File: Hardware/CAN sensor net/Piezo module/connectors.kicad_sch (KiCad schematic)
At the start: 7 parts, among them J1 532610671, J2 532610671, J3 USB_B_Micro, U4 USBLC6-2SC6

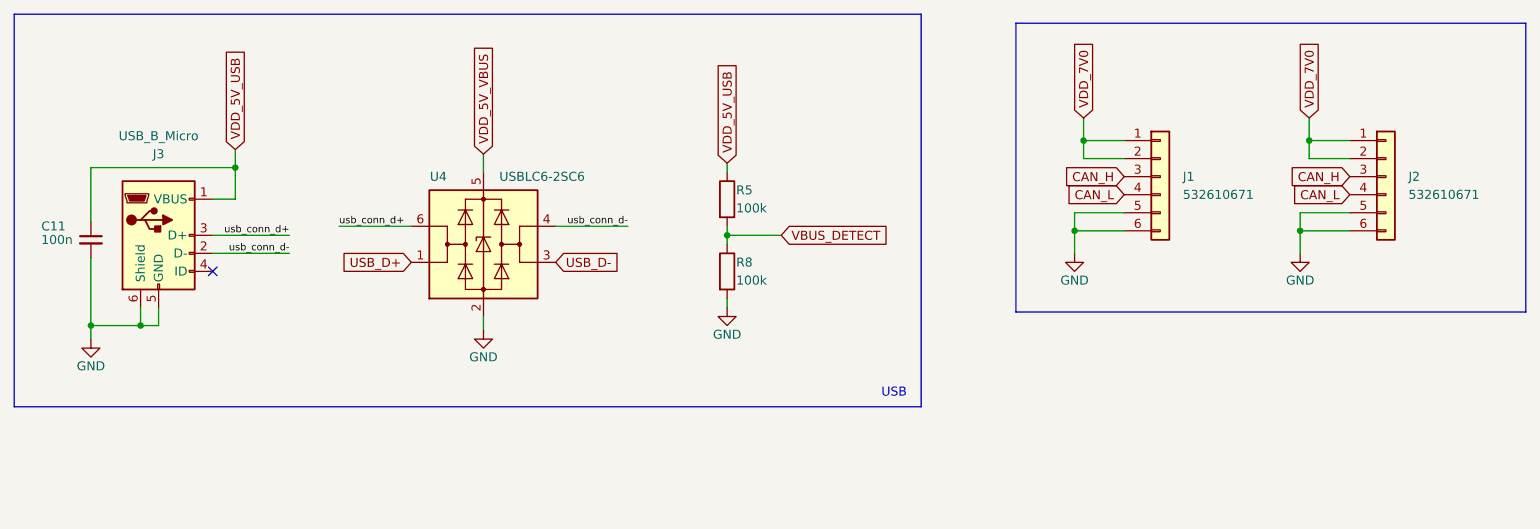
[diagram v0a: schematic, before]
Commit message: Bugfix
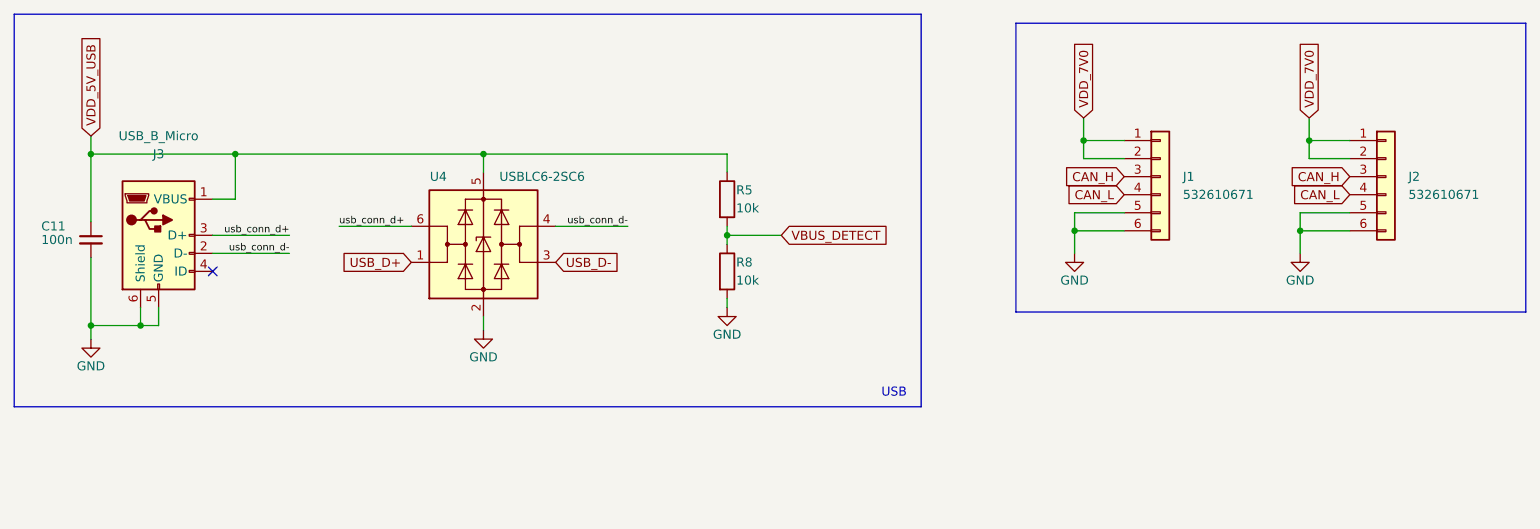
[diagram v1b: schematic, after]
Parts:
- R5, R8: value 100k -> 10k
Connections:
- net VDD_5V_VBUS is gone; now on net VDD_5V_USB: U4.5 (VBUS)
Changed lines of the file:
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@@
 	(paper "A4")
 	(junction
-		(at 52.705 43.815)
+		(at 52.705 41.91)
+		(diameter 0)
+		(color 0 0 0 0)
+	)
+	(junction
+		(at 32.385 41.91)
+		(diameter 0)
+		(color 0 0 0 0)
+	)
+	(junction
+		(at 87.63 41.91)
 		(diameter 0)
 		(color 0 0 0 0)
@@
 	(wire
 		(pts
-			(xy 121.92 43.18) (xy 121.92 44.45)
+			(xy 121.92 41.91) (xy 121.92 44.45)
 		)
 		(stroke
@@
 		)
 	)
+	(wire
+		(pts
+			(xy 52.705 41.91) (xy 87.63 41.91)
+		)
+		(stroke
+			(width 0)
+			(type default)
+		)
+	)
 	(polyline
 		(pts
@@
 	(wire
 		(pts
-			(xy 52.705 48.26) (xy 52.705 43.815)
+			(xy 52.705 41.91) (xy 52.705 48.26)
 		)
 		(stroke
@@
 	(wire
 		(pts
+			(xy 121.92 41.91) (xy 87.63 41.91)
+		)
+		(stroke
+			(width 0)
+			(type default)
+		)
+	)
+	(wire
+		(pts
 			(xy 87.63 64.77) (xy 87.63 66.675)
 		)
@@
 	(wire
 		(pts
-			(xy 52.705 41.275) (xy 52.705 43.815)
+			(xy 32.385 39.37) (xy 32.385 41.91)
 		)
 		(stroke
@@
 	(wire
 		(pts
-			(xy 52.705 43.815) (xy 32.385 43.815)
+			(xy 52.705 41.91) (xy 32.385 41.91)
 		)
 		(stroke
@@
 	(wire
 		(pts
-			(xy 32.385 43.815) (xy 32.385 51.435)
+			(xy 32.385 41.91) (xy 32.385 51.435)
 		)
 		(stroke
@@
 	(global_label "VDD_5V_USB"
 		(shape input)
-		(at 121.92 43.18 90)
+		(at 32.385 39.37 90)
 		(fields_autoplaced yes)
 		(effects
@@
 		)
 		(property "Intersheetrefs" "${INTERSHEET_REFS}"
-			(at 121.92 28.5229 90)
-			(effects
-				(font
-					(size 1.27 1.27)
-				)
-				(justify left)
-				(hide yes)
-			)
-		)
-	)
-	(global_label "VDD_5V_USB"
-		(shape input)
-		(at 52.705 41.275 90)
-		(fields_autoplaced yes)
-		(effects
-			(font
-				(size 1.27 1.27)
-			)
-			(justify left)
-		)
-		(property "Intersheetrefs" "${INTERSHEET_REFS}"
-			(at 52.705 26.6179 90)
-			(effects
-				(font
-					(size 1.27 1.27)
-				)
-				(justify left)
-				(hide yes)
-			)
-		)
-	)
-	(global_label "VDD_5V_VBUS"
-		(shape input)
-		(at 87.63 41.91 90)
-		(fields_autoplaced yes)
-		(effects
-			(font
-				(size 1.27 1.27)
-			)
-			(justify left)
-		)
-		(property "Intersheetrefs" "${INTERSHEET_REFS}"
-			(at 87.7094 26.7364 90)
+			(at 32.385 24.7129 90)
 			(effects
 				(font
@@
 			)
 		)
-		(property "Value" "100k"
+		(property "Value" "10k"
 			(at 123.19 59.69 0)
 			(effects
@@
 			)
 		)
-		(property "Value" "100k"
+		(property "Value" "10k"
 			(at 123.19 49.53 0)
 			(effects

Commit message: updated piezo module
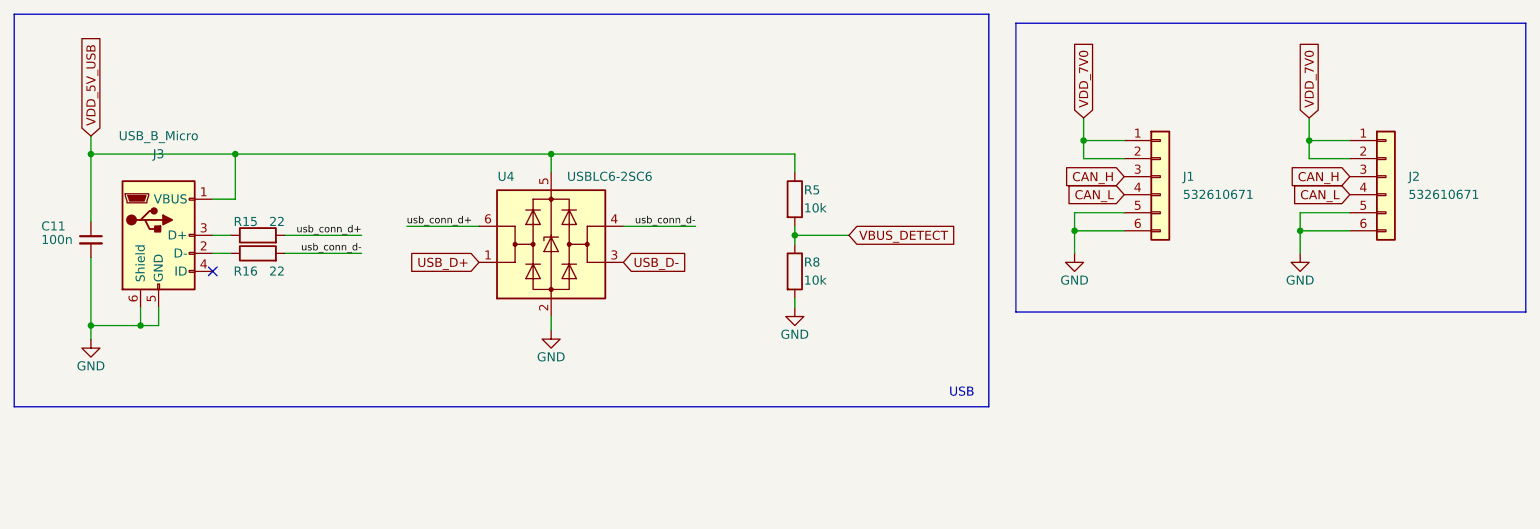
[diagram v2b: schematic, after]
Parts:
- added R15, R16: 22, Resistor_SMD:R_0603_1608Metric, symbol Device:R
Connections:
- net usb_conn_d+: now also R15.2; no longer J3.3 (D+)
- net usb_conn_d-: now also R16.2; no longer J3.2 (D-)
- new net: J3.2 (D-), R16.1
- new net: J3.3 (D+), R15.1
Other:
- moved on the sheet: R5, R8, U4

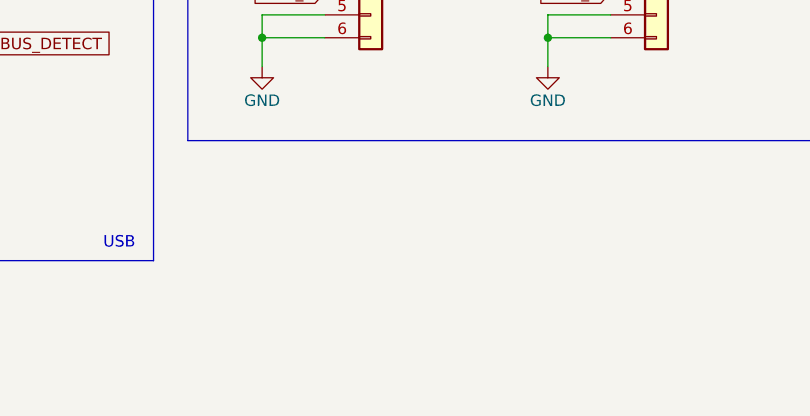
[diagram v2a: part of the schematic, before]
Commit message: added band pass filter to piezo board
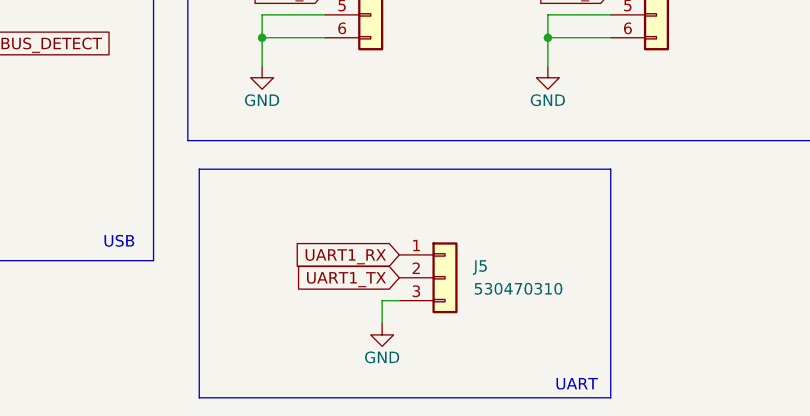
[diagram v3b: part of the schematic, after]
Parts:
- added J5: 530470310, Connector_Molex:Molex_PicoBlade_53261-0371_1x03-1MP_P1.25mm_Horizontal, symbol Connector_Generic:Conn_01x03
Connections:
- net GND: now also J5.3 (Pin_3)
- new net UART1_RX: J5.1 (Pin_1)
- new net UART1_TX: J5.2 (Pin_2)
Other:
- note added: "UART"
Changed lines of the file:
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@@
+		)
+	)
+	(polyline
+		(pts
+			(xy 209.55 67.31) (xy 209.55 92.71)
+		)
+		(stroke
+			(width 0)
+			(type default)
 		)
 	)
@@
 	(wire
 		(pts
+			(xy 186.055 81.915) (xy 184.15 81.915)
+		)
+		(stroke
+			(width 0)
+			(type default)
+		)
+	)
+	(wire
+		(pts
 			(xy 203.835 40.005) (xy 209.55 40.005)
 		)
@@
 	(wire
 		(pts
+			(xy 184.15 81.915) (xy 184.15 84.455)
+		)
+		(stroke
+			(width 0)
+			(type default)
+		)
+	)
+	(wire
+		(pts
 			(xy 203.835 42.545) (xy 203.835 40.005)
 		)
@@
 		)
 	)
+	(polyline
+		(pts
+			(xy 163.83 92.71) (xy 163.83 67.31)
+		)
+		(stroke
+			(width 0)
+			(type default)
+		)
+	)
 	(wire
 		(pts
@@
 		)
 	)
+	(polyline
+		(pts
+			(xy 163.83 92.71) (xy 209.55 92.71)
+		)
+		(stroke
+			(width 0)
+			(type default)
+		)
+	)
 	(wire
 		(pts
@@
 		)
 	)
+	(polyline
+		(pts
+			(xy 163.83 67.31) (xy 209.55 67.31)
+		)
+		(stroke
+			(width 0)
+			(type default)
+		)
+	)
 	(wire
 		(pts
@@
 			(width 0)
 			(type default)
+		)
+	)
+	(text "UART"
+		(exclude_from_sim no)
+		(at 205.74 91.44 0)
+		(effects
+			(font
+				(size 1.27 1.27)
+			)
 		)
 	)
@@
 		)
 	)
+	(global_label "UART1_TX"
+		(shape input)
+		(at 186.055 79.375 180)
+		(fields_autoplaced yes)
+		(effects
+			(font
+				(size 1.27 1.27)
+			)
+			(justify right)
+		)
+		(property "Intersheetrefs" "${INTERSHEET_REFS}"
+			(at 174.0589 79.375 0)
+			(effects
+				(font
+					(size 1.27 1.27)
+				)
+				(justify right)
+				(hide yes)
+			)
+		)
+	)
 	(global_label "VDD_5V_USB"
 		(shape input)
@@
 				)
 				(justify left)
+				(hide yes)
+			)
+		)
+	)
+	(global_label "UART1_RX"
+		(shape input)
+		(at 186.055 76.835 180)
+		(fields_autoplaced yes)
+		(effects
+			(font
+				(size 1.27 1.27)
+			)
+			(justify right)
+		)
+		(property "Intersheetrefs" "${INTERSHEET_REFS}"
+			(at 173.7565 76.835 0)
+			(effects
+				(font
+					(size 1.27 1.27)
+				)
+				(justify right)
 				(hide yes)
 			)
@@
 	)
 	(symbol
+		(lib_name "GND_1")
+		(lib_id "power:GND")
+		(at 184.15 84.455 0)
+		(unit 1)
+		(exclude_from_sim no)
+		(in_bom yes)
+		(on_board yes)
+		(dnp no)
+		(property "Reference" "#PWR019"
+			(at 184.15 90.805 0)
+			(effects
+				(font
+					(size 1.27 1.27)
+				)
+				(hide yes)
+			)
+		)
+		(property "Value" "GND"
+			(at 184.15 88.265 0)
+			(effects
+				(font
+					(size 1.27 1.27)
+				)
+			)
+		)
+		(property "Footprint" ""
+			(at 184.15 84.455 0)
+			(effects
+				(font
+					(size 1.27 1.27)
+				)
+				(hide yes)
+			)
+		)
+		(property "Datasheet" ""
+			(at 184.15 84.455 0)
+			(effects
+				(font
+					(size 1.27 1.27)
+				)
+				(hide yes)
+			)
+		)
+		(property "Description" "Power symbol creates a global label with name \"GND\" , ground"
+			(at 184.15 84.455 0)
+			(effects
+				(font
+					(size 1.27 1.27)
+				)
+				(hide yes)
+			)
+		)
+		(pin "1"
+		)
+		(instances
+			(project "Piezo module"
+				(path "/0a58466e-2312-402a-82c7-7de62fe91dff/33325e08-e21c-439d-a7db-dde9f8ca3ce6"
+					(reference "#PWR019")
+					(unit 1)
+				)
+			)
+		)
+	)
+	(symbol
 		(lib_id "power:GND")
 		(at 97.155 66.675 0)
@@
 					(unit 1)
 				)
+			)
+		)
+	)
+	(symbol
+		(lib_id "Connector_Generic:Conn_01x03")
+		(at 191.135 79.375 0)
+		(unit 1)
+		(exclude_from_sim no)
+		(in_bom yes)
+		(on_board yes)
+		(dnp no)
+		(fields_autoplaced yes)
+		(property "Reference" "J5"
+			(at 194.31 78.1049 0)
+			(effects
+				(font
+					(size 1.27 1.27)
+				)
+				(justify left)
+			)
+		)
+		(property "Value" "530470310"
+			(at 194.31 80.6449 0)
+			(effects
+				(font
+					(size 1.27 1.27)
+				)
+				(justify left)
+			)
+		)
+		(property "Footprint" "Connector_Molex:Molex_PicoBlade_53261-0371_1x03-1MP_P1.25mm_Horizontal"
+			(at 191.135 79.375 0)
+			(effects
+				(font
+					(size 1.27 1.27)
+				)
+				(hide yes)
+			)
+		)
+		(property "Datasheet" "~"
+			(at 191.135 79.375 0)
+			(effects
+				(font
+					(size 1.27 1.27)
+				)
+				(hide yes)
+			)
+		)
+		(property "Description" "Generic connector, single row, 01x03, script generated (kicad-library-utils/schlib/autogen/connector/)"
+			(at 191.135 79.375 0)
+			(effects
+				(font
+					(size 1.27 1.27)
+				)
+				(hide yes)
+			)
+		)
+		(pin "2"
+		)
+		(pin "3"
+		)
+		(pin "1"
+		)
+		(instances
+			(project "Piezo module"
+				(path "/0a58466e-2312-402a-82c7-7de62fe91dff/33325e08-e21c-439d-a7db-dde9f8ca3ce6"
+					(reference "J5")
+					(unit 1)
+				)

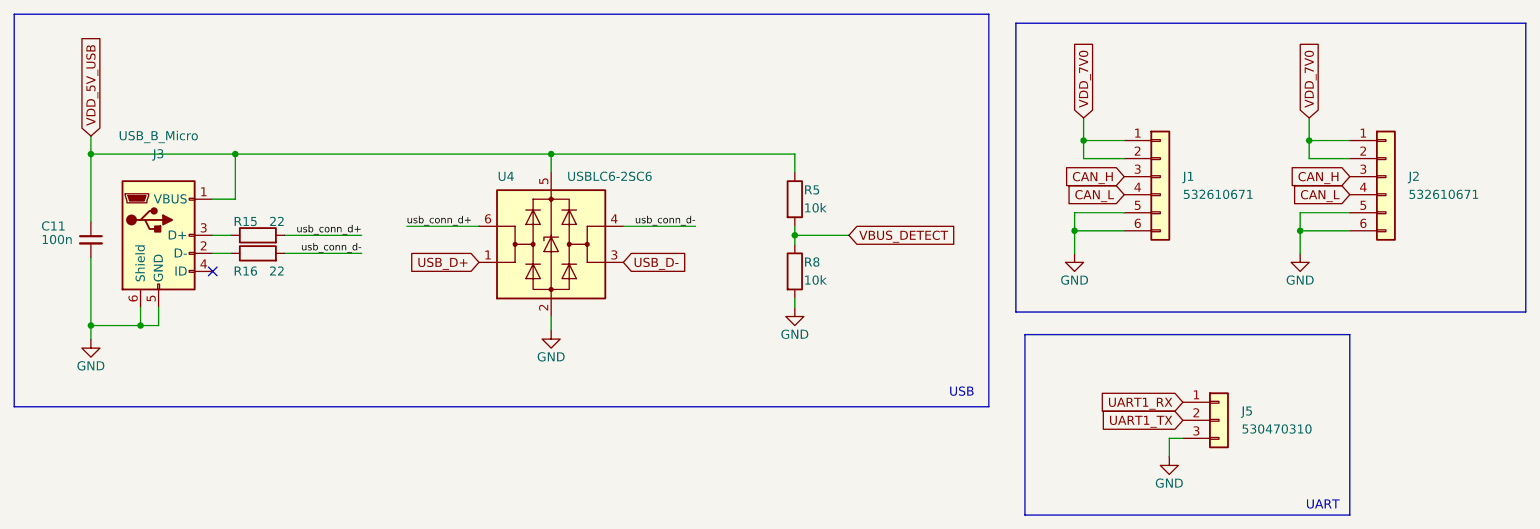
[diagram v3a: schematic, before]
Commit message: updated piezo board schematics
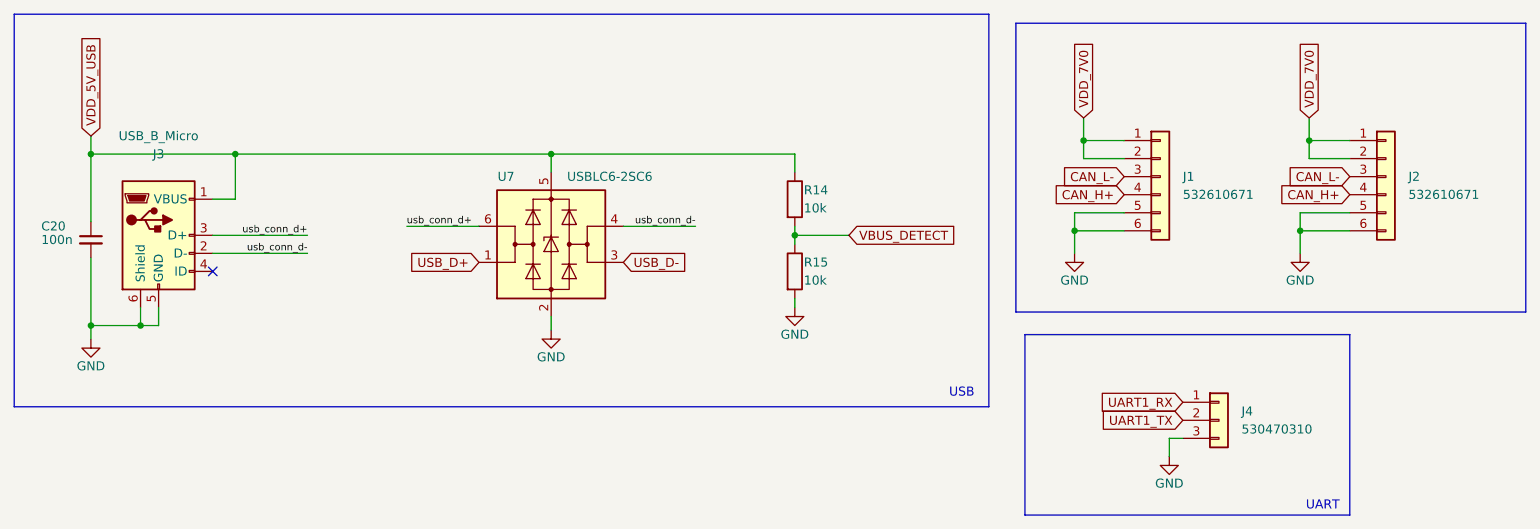
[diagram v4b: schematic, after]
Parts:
- removed R15, R16: 22, Resistor_SMD:R_0603_1608Metric, symbol Device:R
- renumbered C11 to C20, J5 to J4, R5 to R14, R8 to R15, U4 to U7
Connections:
- net usb_conn_d+: now also J3.3 (D+)
- net usb_conn_d-: now also J3.2 (D-)
- net CAN_H renamed CAN_L-
- net CAN_L renamed CAN_H+
